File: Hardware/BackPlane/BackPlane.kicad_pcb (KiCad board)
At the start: 2 copper layers, 150 x 97 mm, 20 parts, among them J1 CAN, J102 i²c, J104 GPIO, J2 Power Harness, J3 CAN, U101 COMPUTER, U102 CARD 0, U103 CARD 1, U104 CARD 2, U105 CARD 3

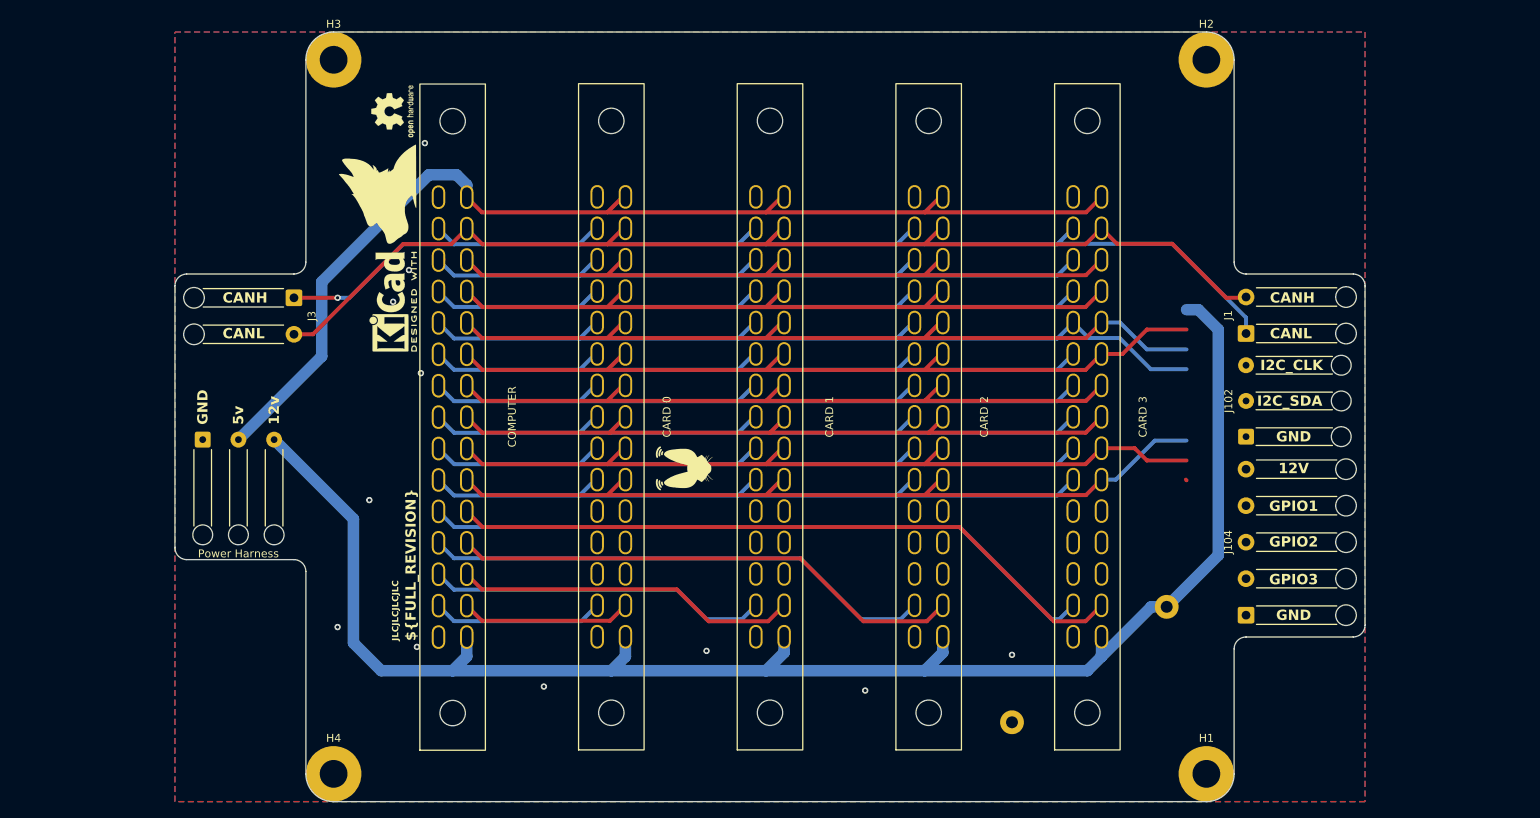
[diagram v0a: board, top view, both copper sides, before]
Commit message: So near to a backplane prototype now
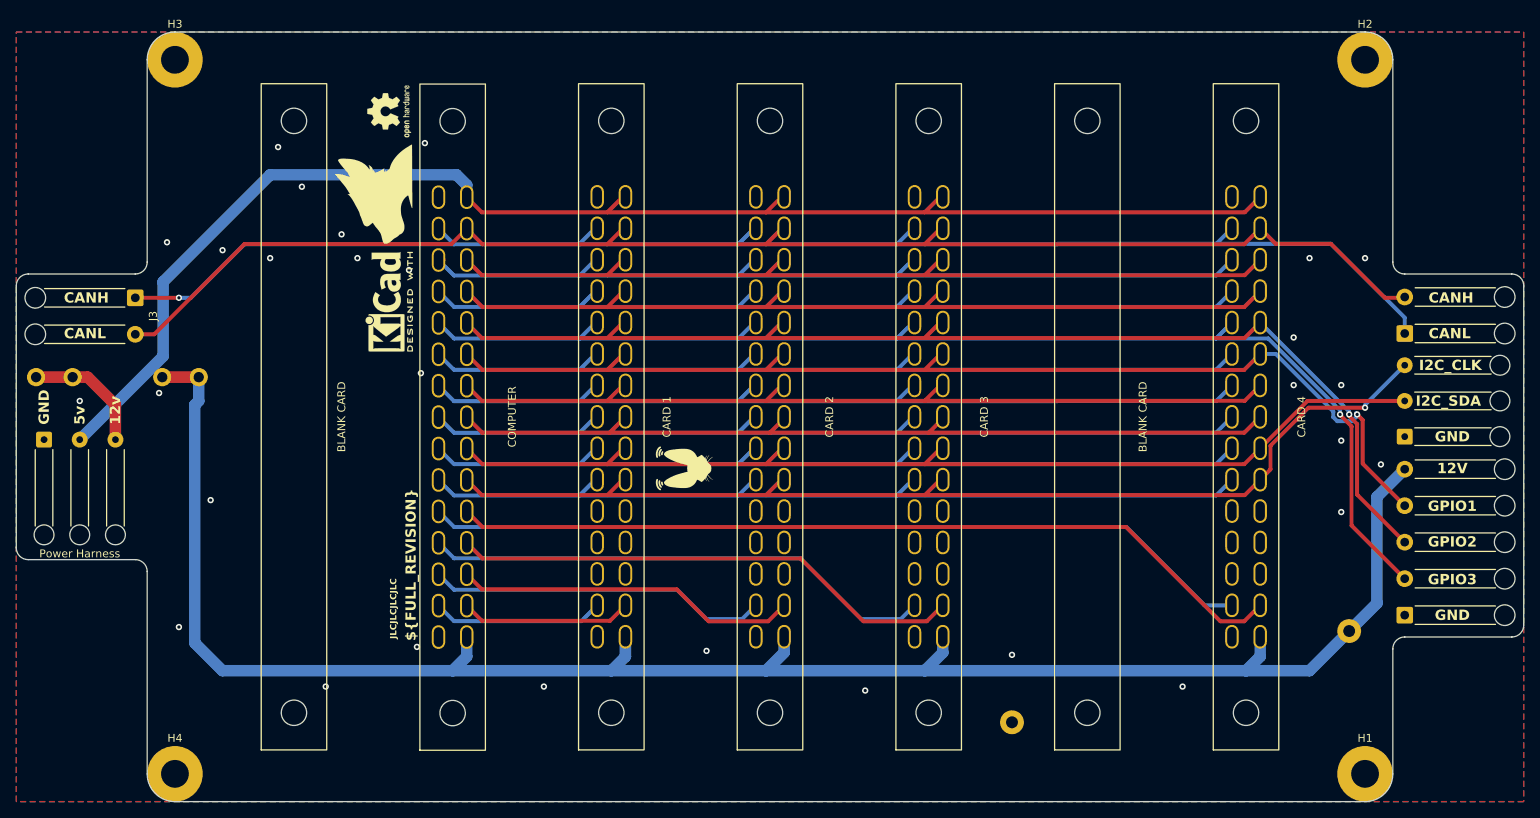
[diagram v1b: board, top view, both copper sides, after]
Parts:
- added F1: Fuse, Fuse:Fuseholder_Littelfuse_100_series_5x20mm, B.Cu at (-72.0, -5.00)
- added REF**: EBM15DSEH, KenwoodFox:EBM15DSEH_Blank, F.Cu at (-60.0, 0.00)
- added REF**: EBM15DSEH, KenwoodFox:EBM15DSEH_Blank, F.Cu at (40.0, 0.00)
- U102: value CARD 0 -> CARD 1
- U103: value CARD 1 -> CARD 2
- U104: value CARD 2 -> CARD 3
- U105: value CARD 3 -> CARD 4
- moved TP101 23.2 mm to (73.0, 27.0)
- moved H1 20.0 mm to (75.0, 45.0)
- moved H2 20.0 mm to (75.0, -45.0)
- moved H3 20.0 mm to (-75.0, -45.0)
- moved H4 20.0 mm to (-75.0, 45.0)
- moved J1 20.0 mm to (80.0, -10.5)
- moved J102 20.0 mm to (80.0, 2.50)
- moved J104 20.0 mm to (80.0, 25.0)
- moved J2 20.0 mm to (-91.5, 2.88)
- moved J3 20.0 mm to (-80.0, -15.0)
- moved U105 20.0 mm to (60.0, 0.00)
- moved LOGO1 0.50 mm to (-50.0, -28.0)
- moved LOGO3 0.50 mm to (-48.0, -38.5)
- moved LOGO5 0.50 mm to (-48.0, -14.5)
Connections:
- J2 pad 3: +12V -> Net-(J2-Pin_3)
- U101 pad 10: /CARD_SEL_3 -> /CARD_SEL_4
- U101 pad 3: /CARD_EN_0 -> /CARD_EN_1
- U101 pad 4: /CARD_SEL_0 -> /CARD_SEL_1
- U101 pad 5: /CARD_EN_1 -> /CARD_EN_2
- U101 pad 6: /CARD_SEL_1 -> /CARD_SEL_2
- U101 pad 7: /CARD_EN_2 -> /CARD_EN_3
- U101 pad 8: /CARD_SEL_2 -> /CARD_SEL_3
- U101 pad 9: /CARD_EN_3 -> /CARD_EN_4
- U102 pad 3: /CARD_EN_0 -> /CARD_EN_1
- U102 pad 4: /CARD_SEL_0 -> /CARD_SEL_1
- U103 pad 3: /CARD_EN_1 -> /CARD_EN_2
- U103 pad 4: /CARD_SEL_1 -> /CARD_SEL_2
- U104 pad 3: /CARD_EN_2 -> /CARD_EN_3
- U104 pad 4: /CARD_SEL_2 -> /CARD_SEL_3
- U105 pad 3: /CARD_EN_3 -> /CARD_EN_4
- U105 pad 4: /CARD_SEL_3 -> /CARD_SEL_4
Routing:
- net /CARD_EN_4: track 0.00 -> 106.6 mm
- net /CARD_SEL_4: track 0.00 -> 104.9 mm
- net /GPIO3: track 107.5 -> 154.8 mm, vias 0 -> 1
- net /GPIO2: track 103.0 -> 146.1 mm, vias 0 -> 1
- net /CANL: track 143.5 -> 183.5 mm
- net /CANH: track 140.1 -> 180.1 mm
- net +5V: track 141.0 -> 181.0 mm
- net /GPIO1: track 103.0 -> 141.9 mm, vias 0 -> 1
- net +12V: track 203.9 -> 237.3 mm
- net /I2C_CLK: track 103.6 -> 137.0 mm, vias 0 -> 1
- net /I2C_SDA: track 102.3 -> 131.7 mm
- net /CARD_EN_1: track 43.3 -> 21.6 mm
- net /CARD_SEL_2: track 64.7 -> 43.1 mm
- net /CARD_EN_3: track 86.6 -> 64.9 mm
- net /CARD_EN_2: track 64.9 -> 43.3 mm
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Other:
- board size 150 x 97 mm -> 190 x 97 mm
- board text added: "BLANK CARD"
- board text removed: "+12v"
- board text removed: "SCL"
- board text removed: "SDA"
